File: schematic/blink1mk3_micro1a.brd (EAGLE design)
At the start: 14.9 x 9.6 mm, 15 parts, among them U1 EFM32HG309F64G, X2 USBPCB2

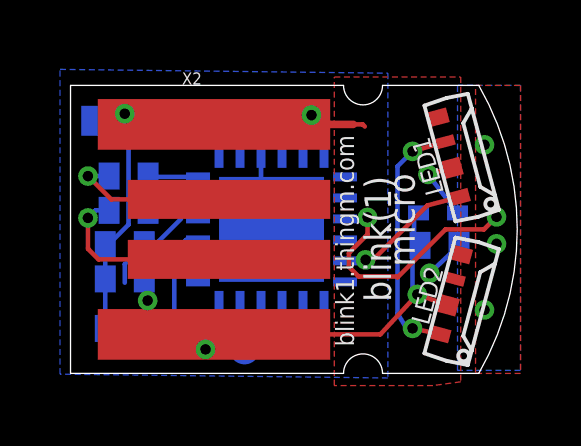
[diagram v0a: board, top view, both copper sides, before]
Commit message: add more micro ideas
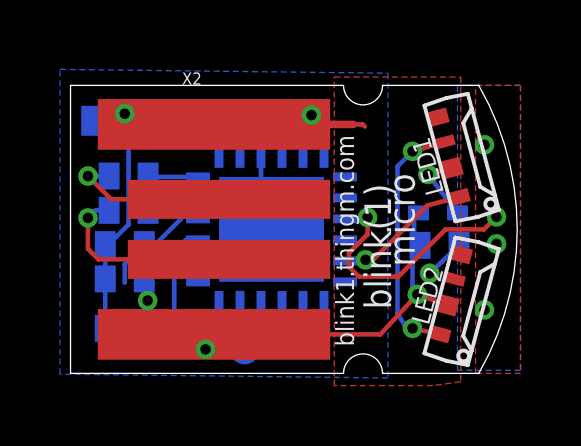
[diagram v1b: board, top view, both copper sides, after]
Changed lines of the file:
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@@
 <plain>
 <text x="8.1486" y="-3.8999" size="0.6096" layer="21" ratio="12" rot="SR90">blink1.thingm.com</text>
-<text x="9.385" y="-2.412" size="0.889" layer="21" ratio="12" rot="R90">blink(1)</text>
+<text x="9.385" y="-2.666" size="0.889" layer="21" ratio="12" rot="R90">blink(1)</text>
 <text x="9.209" y="-3.983" size="0.6096" layer="22" ratio="10" rot="MR90">blink1mk3micro1a</text>
 <rectangle x1="8.3407" y1="12.3031" x2="10.2457" y2="12.3095" layer="200"/>
